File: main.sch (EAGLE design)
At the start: 46 parts, among them IC1 ATTINY13A-SSH, IC2 TP4056-42-ESOP8, IC3 LM27313XMFX_NOPB, IC4 TPL5110DDCT, IC5 ATTINY13A-SSH, T1A 2N4401, T1B NPN, X1 MINI-USB-UX60A-MB-5ST, X2 332-02

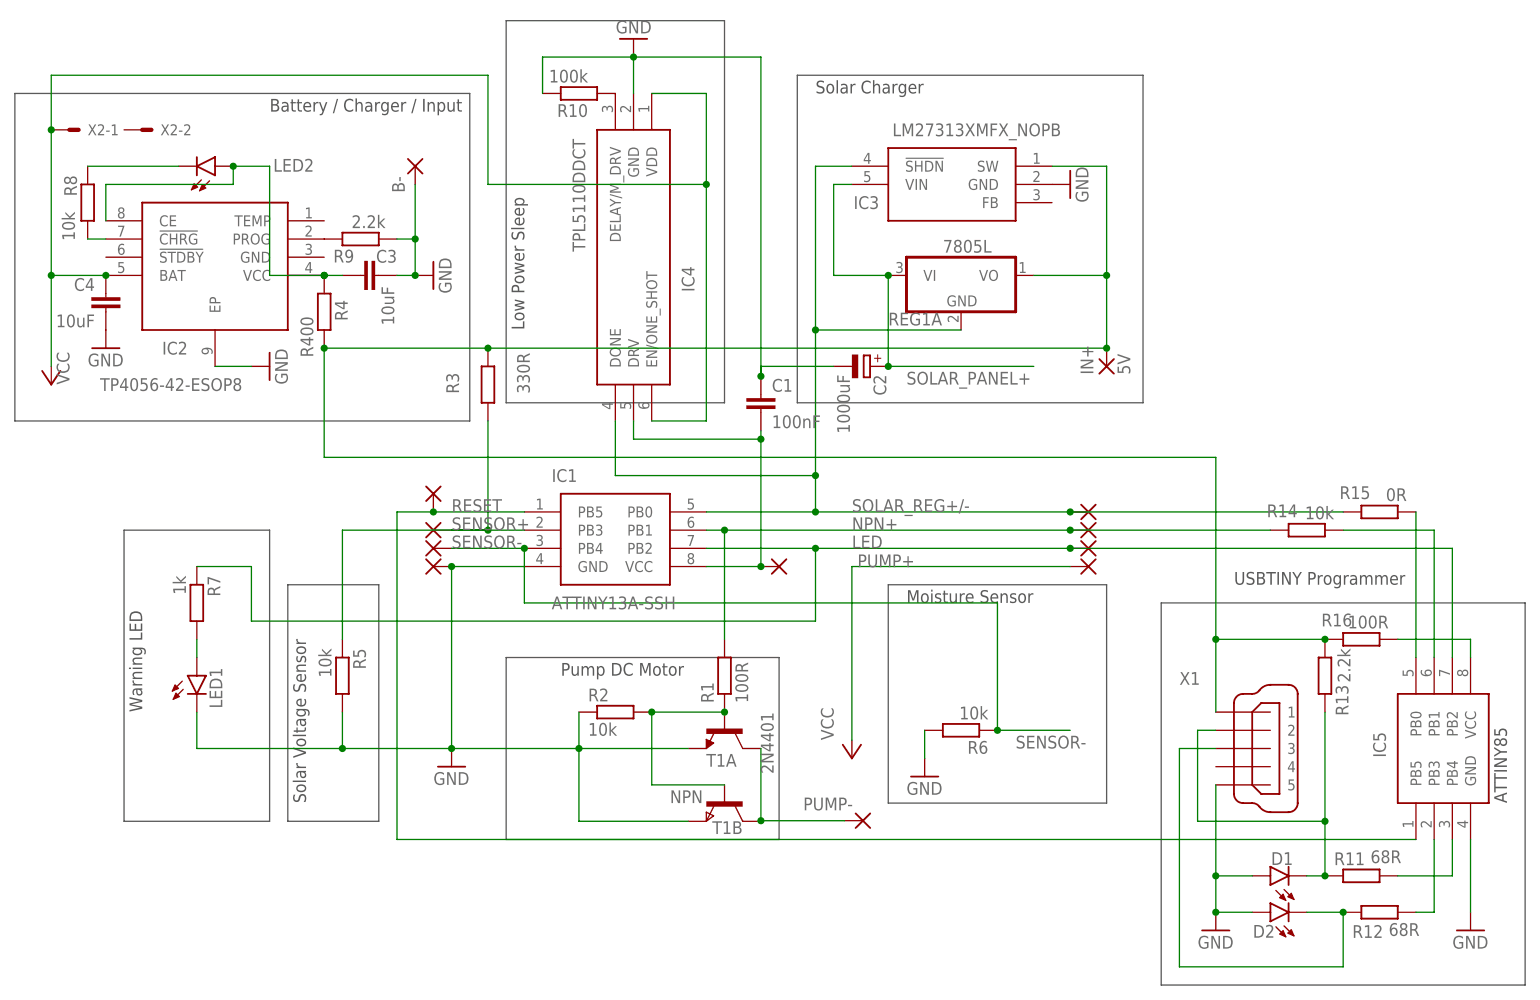
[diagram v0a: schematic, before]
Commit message: updates
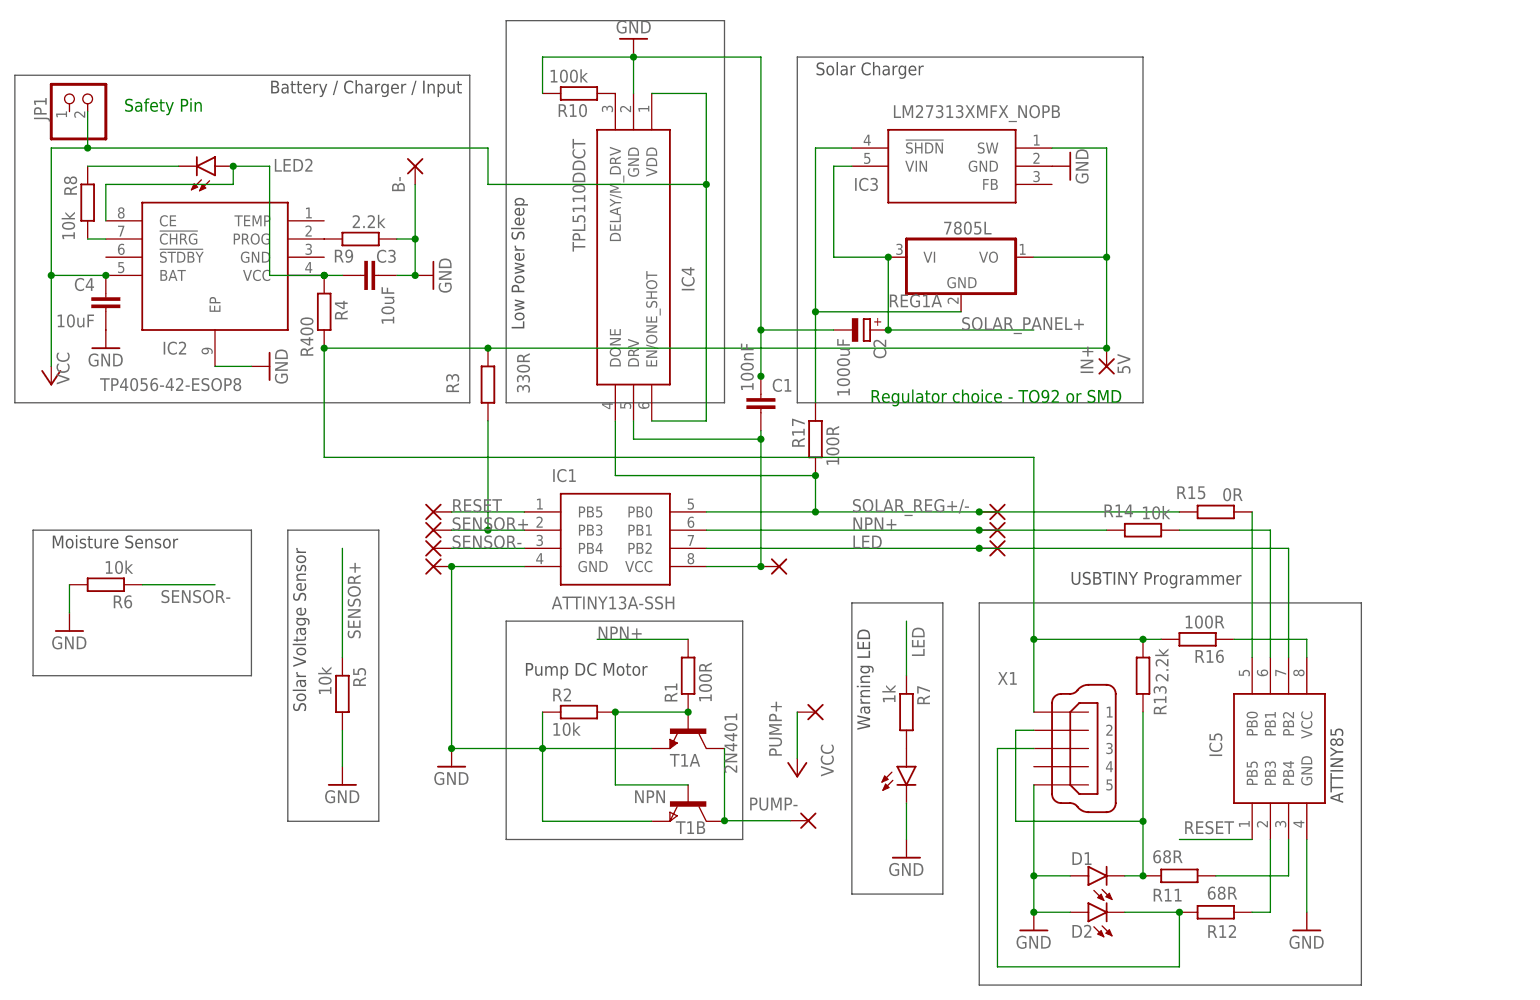
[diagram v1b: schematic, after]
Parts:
- removed X2: 332-02, con-garry:332-02
- added JP1: (no value), pinhead:PINHD-1X2/90
- added R17: 100R, resistor:R-EU_R0603
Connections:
- new net N$18: IC3.!SHDN, R17.2, REG1A.GND
- net SOLAR_REG+/-: now also R17.1; no longer IC3.!SHDN, REG1A.GND
- net VCC: now also JP1.2; no longer X2-1.S
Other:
- note added: "Regulator choice - TO92 or SMD"
- note added: "Safety Pin"
- moved on the sheet: C2, D1, D2, IC3, IC5, PUMP+, PUMP-, R1, R11, R12, R13, R14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
